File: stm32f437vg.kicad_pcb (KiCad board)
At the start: 2 copper layers, 106.9 x 74.1 mm, 51 parts, among them P1 CONN_BOOT0, P10 CONN_01X17, P12 Power 3.3V, P13 CONN_01X21, P14 USB_OTG, P15 CONN_02X03, P16 USB_A, P17 CONN_01X13, P18 CONN_01X05, P19 CONN_01X13, P2 CONN_01X05, P20 CONN_01X03, P21 CONN_01X20, P22 PA3, P3 CONN_XTAL, P4 swd, P5 CONN_01X05, P6 CONN_01X04, P7 CONN_01X04, P8 CONN_01X02, P9 CONN_01X04, SW1 SW_PUSH, SW2 SW_PUSH, U1 STM32F437VG, U2 LM1117-3.3, Y1 Crystal

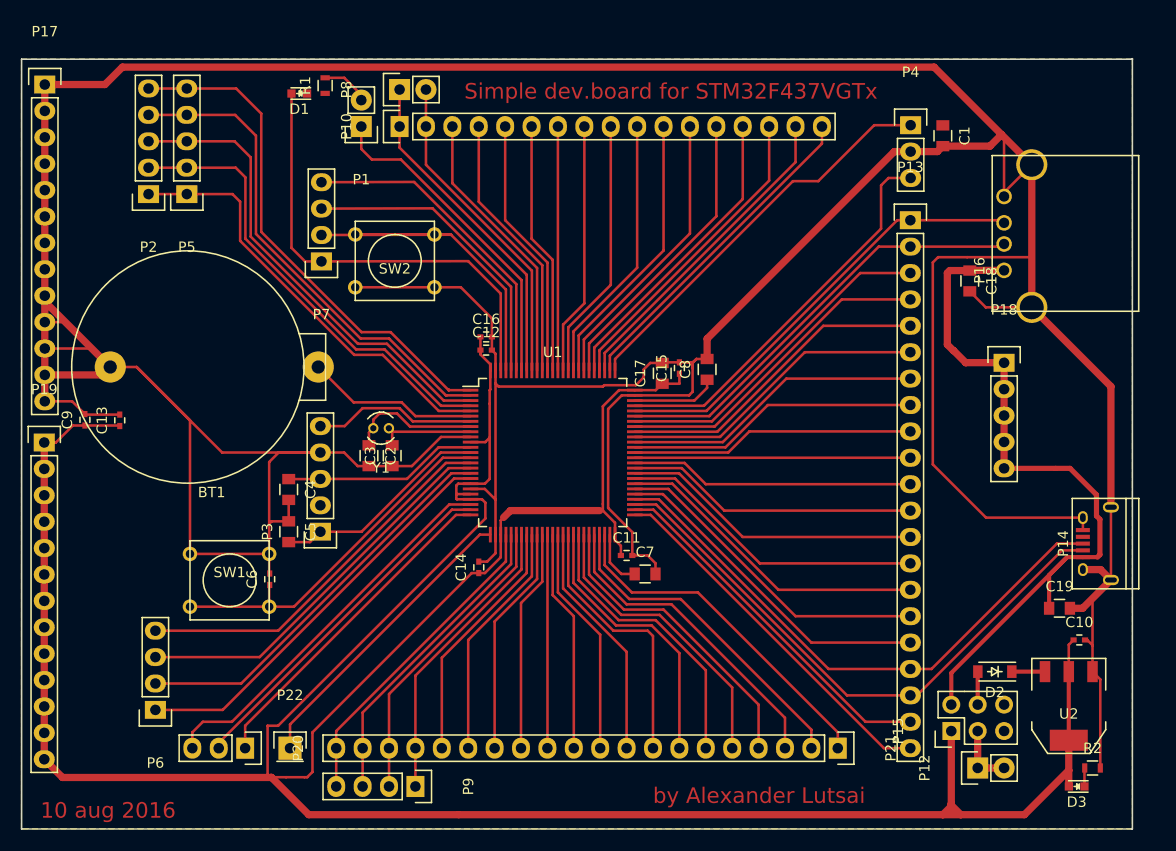
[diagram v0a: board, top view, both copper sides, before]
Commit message: final fix
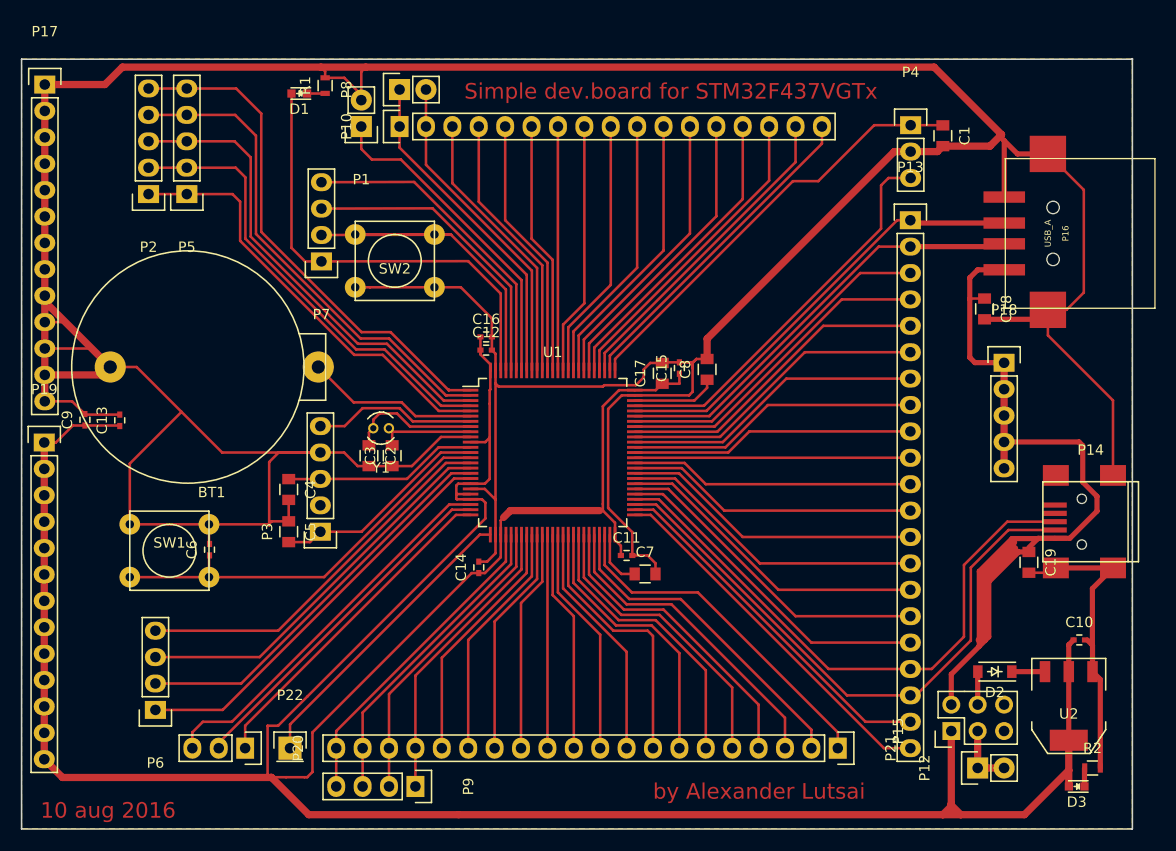
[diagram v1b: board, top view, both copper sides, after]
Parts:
- P14: footprint Connect:USB_Micro-B -> Connect:USB_Mini-B
- P16: footprint Connect:USB_A -> kicad-libraries1:USB-A-SMT-8231-PEG
- moved C6 6.45 mm to (107.7, 112.5)
- moved SW1 6.45 mm to (103.8, 112.6)
- moved P16 5.52 mm to (188.4, 82.0)
- moved C19 5.31 mm to (186.5, 113.7), turned to 270 degrees
- moved C18 3.05 mm to (182.3, 89.3)
- moved P14 2.26 mm to (192.5, 109.8), turned to 180 degrees
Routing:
- net GND: track 639.1 -> 549.2 mm
- net +5V: track 86.4 -> 107.3 mm
- net Net-(C6-Pad1): track 35.0 -> 39.7 mm
- net Net-(C1-Pad1): track 38.9 -> 42.0 mm
- net Net-(P13-Pad19): track 56.5 -> 59.4 mm
- net Net-(P13-Pad18): track 54.9 -> 57.1 mm
- net Net-(D1-Pad1): track 0.00 -> 1.74 mm
